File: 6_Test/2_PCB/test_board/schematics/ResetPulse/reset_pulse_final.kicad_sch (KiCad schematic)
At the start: 3 parts

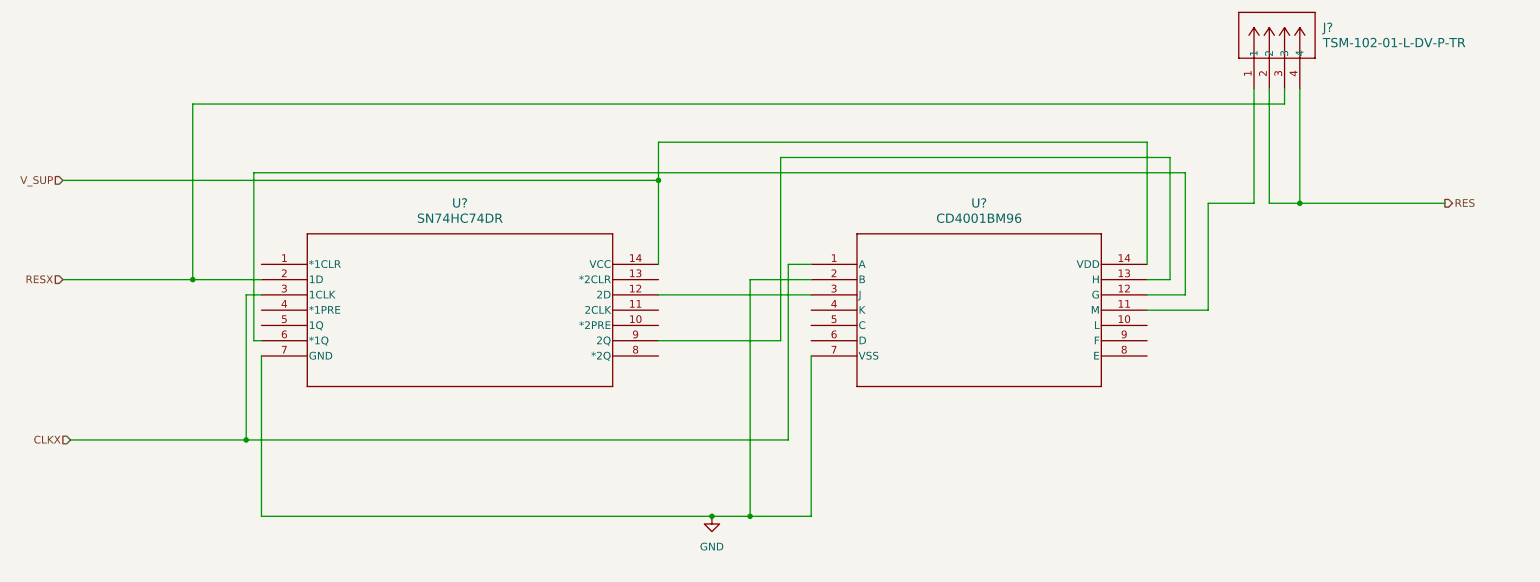
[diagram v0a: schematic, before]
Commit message: Corrections to schematic 11_20_24
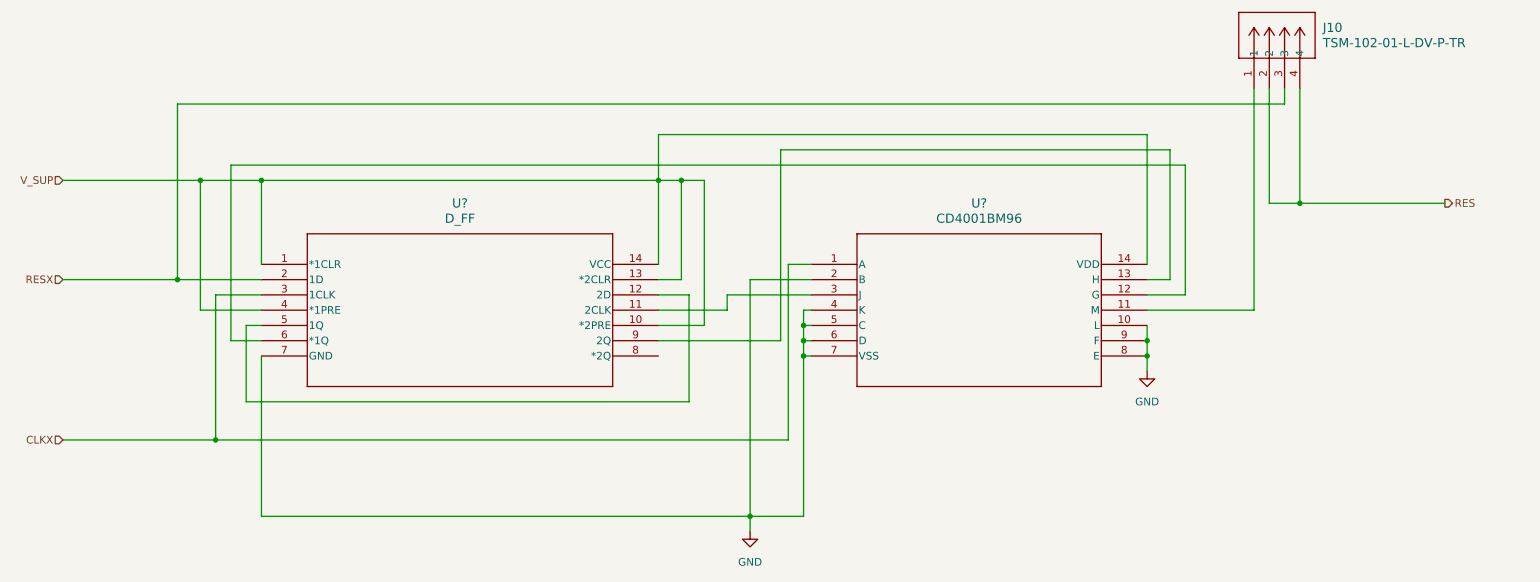
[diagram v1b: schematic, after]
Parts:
- U?: footprint D14 -> nor_gate:nor_gate_D14
- U?: value SN74HC74DR -> D_FF
- gave numbers to parts that had none: 1
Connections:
- net GND: now also U?.10 (L), U?.4 (K), U?.5 (C), U?.6 (D), U?.8 (E), U?.9 (F)
- net V_SUP: now also U?.1 (*1CLR), U?.10 (*2PRE), U?.13 (*2CLR), U?.4 (*1PRE)
- net at U?.3 (J): now also U?.11 (2CLK); no longer U?.12 (2D)
- net at U?.5 (1Q): now also U?.12 (2D)
